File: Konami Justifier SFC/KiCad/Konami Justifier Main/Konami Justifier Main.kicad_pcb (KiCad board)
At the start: 4 copper layers, 25.2 x 50 mm, 21 parts, among them J1 RJ12, J3 Conn_01x06_Socket, U1 74VHC9164FT

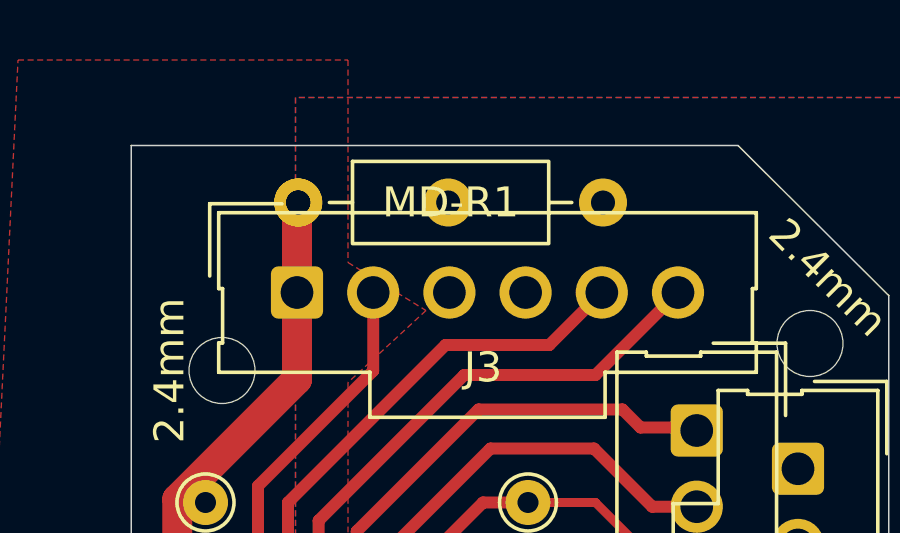
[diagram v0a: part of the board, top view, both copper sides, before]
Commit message: Add files via upload
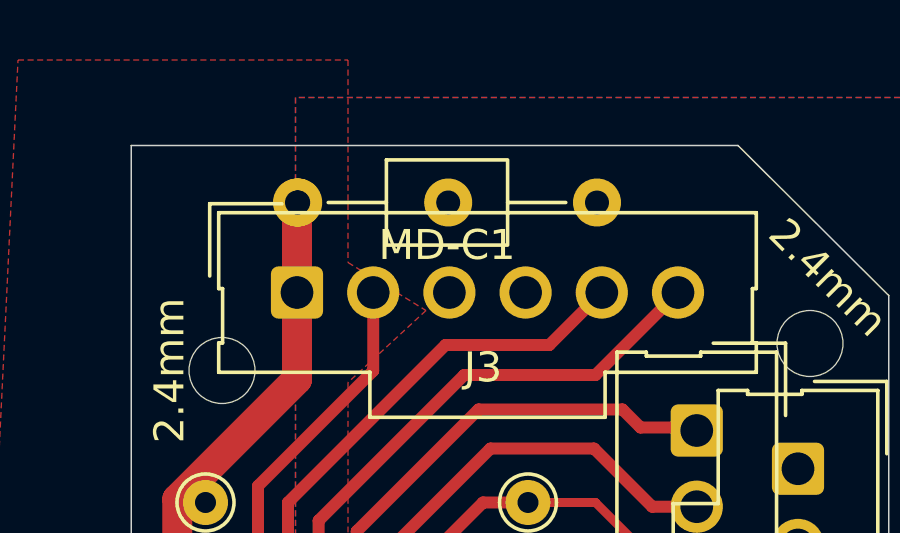
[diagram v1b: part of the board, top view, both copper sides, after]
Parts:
- removed MD-R1: 93 Ohm 1%, Resistor_THT:R_Axial_DIN0207_L6.3mm_D2.5mm_P10.16mm_Horizontal
- added MD-C1: 100nF, Capacitor_THT:C_Axial_L3.8mm_D2.6mm_P10.00mm_Horizontal, F.Cu at (145.3, 78.5)
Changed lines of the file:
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@@
 		(property ki_fp_filters "Pin* Test*")
 		(sheetname "/")
-		(sheetfile "Konami Justifier 02.kicad_sch")
+		(sheetfile "Konami Justifier Main.kicad_sch")
 		(attr exclude_from_pos_files)
 		(fp_circle
@@
 		(property ki_fp_filters "Pin* Test*")
 		(sheetname "/")
-		(sheetfile "Konami Justifier 02.kicad_sch")
+		(sheetfile "Konami Justifier Main.kicad_sch")
 		(attr exclude_from_pos_files)
 		(fp_circle
@@
 		(property ki_fp_filters "6P6C* RJ12* RJ18* RJ25*")
 		(sheetname "/")
-		(sheetfile "Konami Justifier 02.kicad_sch")
+		(sheetfile "Konami Justifier Main.kicad_sch")
 		(attr through_hole)
 		(fp_line
@@
 		(embedded_fonts no)
 	)
-	(footprint "Resistor_THT:R_Axial_DIN0207_L6.3mm_D2.5mm_P10.16mm_Horizontal"
-		(layer "F.Cu")
-		(at 145.34 78.5)
-		(descr "Resistor, Axial_DIN0207 series, Axial, Horizontal, pin pitch=10.16mm, 0.25W = 1/4W, length*diameter=6.3*2.5mm^2, http://cdn-reichelt.de/documents/datenblatt/B400/1_4W%23YAG.pdf")
-		(tags "Resistor Axial_DIN0207 series Axial Horizontal pin pitch 10.16mm 0.25W = 1/4W length 6.3mm diameter 2.5mm")
-		(property "Reference" "MD-R1"
-			(at 5.08 0 0)
-			(layer "F.SilkS")
-			(effects
-				(font
-					(size 1 1)
-					(thickness 0.15)
-				)
-			)
-		)
-		(property "Value" "93 Ohm 1%"
-			(at 5.08 2.37 0)
-			(layer "F.Fab")
-			(effects
-				(font
-					(size 1 1)
-					(thickness 0.15)
-				)
-			)
-		)
-		(property "Datasheet" "~"
-			(at 0 0 0)
-			(layer "F.Fab")
-			(hide yes)
-			(effects
-				(font
-					(size 1.27 1.27)
-					(thickness 0.15)
-				)
-			)
-		)
-		(property "Description" "Resistor"
-			(at 0 0 0)
-			(layer "F.Fab")
-			(hide yes)
-			(effects
-				(font
-					(size 1.27 1.27)
-					(thickness 0.15)
-				)
-			)
-		)
-		(property ki_fp_filters "R_*")
-		(sheetname "/")
-		(sheetfile "Konami Justifier 02.kicad_sch")
-		(attr through_hole)
-		(fp_line
-			(start 1.04 0)
-			(end 1.81 0)
-			(stroke
-				(width 0.12)
-				(type solid)
-			)
-			(layer "F.SilkS")
-		)
-		(fp_line
-			(start 9.12 0)
-			(end 8.35 0)
-			(stroke
-				(width 0.12)
-				(type solid)
-			)
-			(layer "F.SilkS")
-		)
-		(fp_rect
-			(start 1.81 -1.37)
-			(end 8.35 1.37)
-			(stroke
-				(width 0.12)
-				(type solid)
-			)
-			(fill no)
-			(layer "F.SilkS")
-		)
-		(fp_rect
-			(start -1.05 -1.5)
-			(end 11.21 1.5)
-			(stroke
-				(width 0.05)
-				(type solid)
-			)
-			(fill no)
-			(layer "F.CrtYd")
-		)
-		(fp_line
-			(start 0 0)
-			(end 1.93 0)
-			(stroke
-				(width 0.1)
-				(type solid)
-			)
-			(layer "F.Fab")
-		)
-		(fp_line
-			(start 10.16 0)
-			(end 8.23 0)
-			(stroke
-				(width 0.1)
-				(type solid)
-			)
-			(layer "F.Fab")
-		)
-		(fp_rect
-			(start 1.93 -1.25)
-			(end 8.23 1.25)
-			(stroke
-				(width 0.1)
-				(type solid)
-			)
-			(fill no)
-			(layer "F.Fab")
-		)
-		(fp_text user "${REFERENCE}"
-			(at 5.08 0 0)
-			(layer "F.Fab")
-			(effects
-				(font
-					(size 1 1)
-					(thickness 0.15)
-				)
-			)
-		)
-		(pad "1" thru_hole circle
-			(at 0 0)
-			(size 1.6 1.6)
-			(drill 0.8)
-			(layers "*.Cu" "*.Mask")
-			(remove_unused_layers no)
-			(net 6 "+5V")
-			(pintype "passive")
-		)
-		(pad "2" thru_hole circle
-			(at 10.16 0)
-			(size 1.6 1.6)
-			(drill 0.8)
-			(layers "*.Cu" "*.Mask")
-			(remove_unused_layers no)
-			(net 5 "GND")
-			(pintype "passive")
-		)
-		(embedded_fonts no)
-		(model "${KICAD9_3DMODEL_DIR}/Resistor_THT.3dshapes/R_Axial_DIN0207_L6.3mm_D2.5mm_P10.16mm_Horizontal.step"
-			(offset
-				(xyz 0 0 0)
-			)
-			(scale
-				(xyz 1 1 1)
-			)
-			(rotate
-				(xyz 0 0 0)
-			)
-		)
-	)
 	(footprint "Connector_Molex:Molex_SL_171971-0006_1x06_P2.54mm_Vertical"
 		(layer "F.Cu")
@@
 		(property ki_fp_filters "Connector*:*_1x??_*")
 		(sheetname "/")
-		(sheetfile "Konami Justifier 02.kicad_sch")
+		(sheetfile "Konami Justifier Main.kicad_sch")
 		(attr through_hole)
 		(fp_line
@@
 		(property ki_fp_filters "Pin* Test*")
 		(sheetname "/")
-		(sheetfile "Konami Justifier 02.kicad_sch")
+		(sheetfile "Konami Justifier Main.kicad_sch")
 		(attr exclude_from_pos_files)
 		(fp_circle
@@
 		(property ki_fp_filters "Connector*:*_1x??_*")
 		(sheetname "/")
-		(sheetfile "Konami Justifier 02.kicad_sch")
+		(sheetfile "Konami Justifier Main.kicad_sch")
 		(attr through_hole)
 		(fp_circle
@@
 		)
 	)
+	(footprint "Capacitor_THT:C_Axial_L3.8mm_D2.6mm_P10.00mm_Horizontal"
+		(layer "F.Cu")
+		(at 145.3 78.5)
+		(descr "C, Axial series, Axial, Horizontal, pin pitch=10mm, length*diameter=3.8*2.6mm^2, http://www.vishay.com/docs/45231/arseries.pdf")
+		(tags "C Axial series Axial Horizontal pin pitch 10mm  length 3.8mm diameter 2.6mm")
+		(property "Reference" "MD-C1"
+			(at 5 1.42 0)
+			(layer "F.SilkS")
+			(effects
+				(font
+					(size 1 1)
+					(thickness 0.15)
+				)
+			)
+		)
+		(property "Value" "100nF"
+			(at 5 2.42 0)
+			(layer "F.Fab")
+			(effects
+				(font
+					(size 1 1)
+					(thickness 0.15)
+				)
+			)
+		)
+		(property "Datasheet" "~"
+			(at 0 0 0)
+			(layer "F.Fab")
+			(hide yes)
+			(effects
+				(font
+					(size 1.27 1.27)
+					(thickness 0.15)
+				)
+			)
+		)
+		(property "Description" "Unpolarized capacitor"
+			(at 0 0 0)
+			(layer "F.Fab")
+			(hide yes)
+			(effects
+				(font
+					(size 1.27 1.27)
+					(thickness 0.15)
+				)
+			)
+		)
+		(property ki_fp_filters "C_*")
+		(sheetname "/")
+		(sheetfile "Konami Justifier Main.kicad_sch")
+		(attr through_hole)
+		(fp_line
+			(start 1.04 0)
+			(end 2.98 0)
+			(stroke
+				(width 0.12)
+				(type solid)
+			)
+			(layer "F.SilkS")
+		)
+		(fp_line
+			(start 8.96 0)
+			(end 7.02 0)
+			(stroke
+				(width 0.12)
+				(type solid)
+			)
+			(layer "F.SilkS")
+		)
+		(fp_rect
+			(start 2.98 -1.42)
+			(end 7.02 1.42)
+			(stroke
+				(width 0.12)
+				(type solid)
+			)
+			(fill no)
+			(layer "F.SilkS")
+		)
+		(fp_rect
+			(start -1.05 -1.55)
+			(end 11.05 1.55)
+			(stroke
+				(width 0.05)
+				(type solid)
+			)
+			(fill no)
+			(layer "F.CrtYd")
+		)
+		(fp_line
+			(start 0 0)
+			(end 3.1 0)
+			(stroke
+				(width 0.1)
+				(type solid)
+			)
+			(layer "F.Fab")
+		)
+		(fp_line
+			(start 10 0)
+			(end 6.9 0)
+			(stroke
+				(width 0.1)
+				(type solid)
+			)
+			(layer "F.Fab")
+		)
+		(fp_rect
+			(start 3.1 -1.3)
+			(end 6.9 1.3)
+			(stroke
+				(width 0.1)
+				(type solid)
+			)
+			(fill no)
+			(layer "F.Fab")
+		)
+		(fp_text user "${REFERENCE}"
+			(at 5 0 0)
+			(layer "F.Fab")
+			(effects
+				(font
+					(size 0.76 0.76)
+					(thickness 0.114)
+				)
+			)
+		)
+		(pad "1" thru_hole circle
+			(at 0 0)
+			(size 1.6 1.6)
+			(drill 0.8)
+			(layers "*.Cu" "*.Mask")
+			(remove_unused_layers no)
+			(net 6 "+5V")
+			(pintype "passive")
+		)
+		(pad "2" thru_hole circle
+			(at 10 0)
+			(size 1.6 1.6)
+			(drill 0.8)
+			(layers "*.Cu" "*.Mask")
+			(remove_unused_layers no)
+			(net 5 "GND")
+			(pintype "passive")
+		)
+		(embedded_fonts no)
+		(model "${KICAD9_3DMODEL_DIR}/Capacitor_THT.3dshapes/C_Axial_L3.8mm_D2.6mm_P10.00mm_Horizontal.step"
+			(offset
+				(xyz 0 0 0)
+			)
+			(scale
+				(xyz 1 1 1)
+			)
+			(rotate
+				(xyz 0 0 0)
+			)
+		)
+	)
 	(footprint "TestPoint:TestPoint_THTPad_D1.5mm_Drill0.7mm"
 		(layer "F.Cu")
@@
 		(property ki_fp_filters "Pin* Test*")
 		(sheetname "/")
-		(sheetfile "Konami Justifier 02.kicad_sch")
+		(sheetfile "Konami Justifier Main.kicad_sch")
 		(attr exclude_from_pos_files)
 		(fp_circle
@@
 		(property ki_fp_filters "Pin* Test*")
 		(sheetname "/")
-		(sheetfile "Konami Justifier 02.kicad_sch")
+		(sheetfile "Konami Justifier Main.kicad_sch")
 		(attr exclude_from_pos_files)
 		(fp_circle
@@
 		(property ki_fp_filters "Pin* Test*")
 		(sheetname "/")
-		(sheetfile "Konami Justifier 02.kicad_sch")
+		(sheetfile "Konami Justifier Main.kicad_sch")
 		(attr exclude_from_pos_files)
 		(fp_circle
@@
 		(property ki_fp_filters "Connector*:*_1x??_*")
 		(sheetname "/")
-		(sheetfile "Konami Justifier 02.kicad_sch")
+		(sheetfile "Konami Justifier Main.kicad_sch")
 		(attr through_hole)
 		(fp_line
@@
 		(property ki_fp_filters "R_*")
 		(sheetname "/")
-		(sheetfile "Konami Justifier 02.kicad_sch")
+		(sheetfile "Konami Justifier Main.kicad_sch")
 		(attr through_hole)
 		(fp_line
@@
 		(property ki_fp_filters "Connector*:*_1x??_*")
 		(sheetname "/")
-		(sheetfile "Konami Justifier 02.kicad_sch")
+		(sheetfile "Konami Justifier Main.kicad_sch")
 		(attr through_hole)
 		(fp_line
@@
 		(property ki_fp_filters "TSSOP*4.4x5mm*P0.65mm*")
 		(sheetname "/")
-		(sheetfile "Konami Justifier 02.kicad_sch")
+		(sheetfile "Konami Justifier Main.kicad_sch")
 		(attr smd)
 		(fp_line
@@
 		(property ki_fp_filters "R_*")
 		(sheetname "/")
-		(sheetfile "Konami Justifier 02.kicad_sch")
+		(sheetfile "Konami Justifier Main.kicad_sch")
 		(attr through_hole)
 		(fp_line
@@
 		(property ki_fp_filters "C_*")
 		(sheetname "/")
-		(sheetfile "Konami Justifier 02.kicad_sch")
+		(sheetfile "Konami Justifier Main.kicad_sch")
 		(attr through_hole)
 		(fp_circle
@@
 		(property ki_fp_filters "C_*")
 		(sheetname "/")
-		(sheetfile "Konami Justifier 02.kicad_sch")
+		(sheetfile "Konami Justifier Main.kicad_sch")
 		(attr through_hole)
 		(fp_line
@@
 		(property ki_fp_filters "C_*")
 		(sheetname "/")
-		(sheetfile "Konami Justifier 02.kicad_sch")
+		(sheetfile "Konami Justifier Main.kicad_sch")
 		(attr through_hole)
 		(fp_line
